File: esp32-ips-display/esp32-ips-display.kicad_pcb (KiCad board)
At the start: 2 copper layers, 25 parts, among them J1 Conn_01x02_Pin, P1 USB_C_Plug_USB2.0, Q1 NPN, Q2 NPN, U1 ESP32-S3-WROOM-1, U2 CH340C, U3 AMS1117-3.3

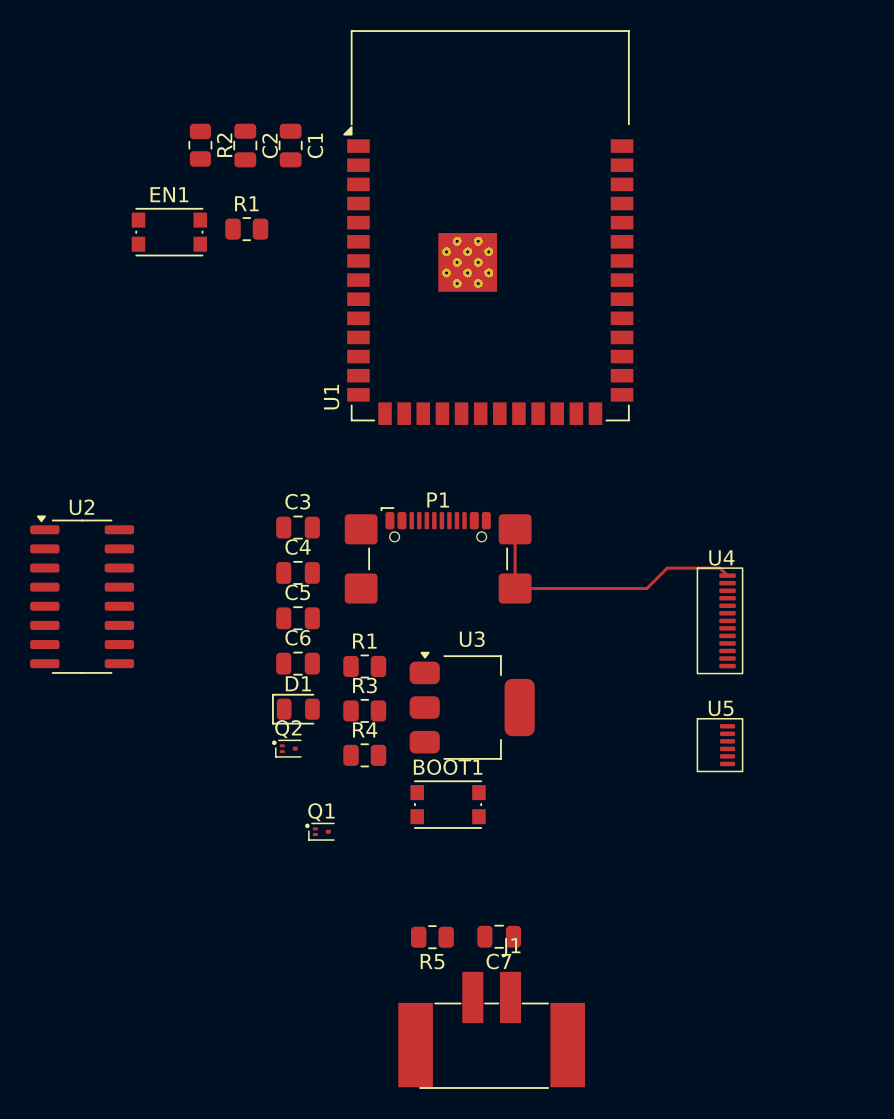
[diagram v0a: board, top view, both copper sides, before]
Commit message: JH
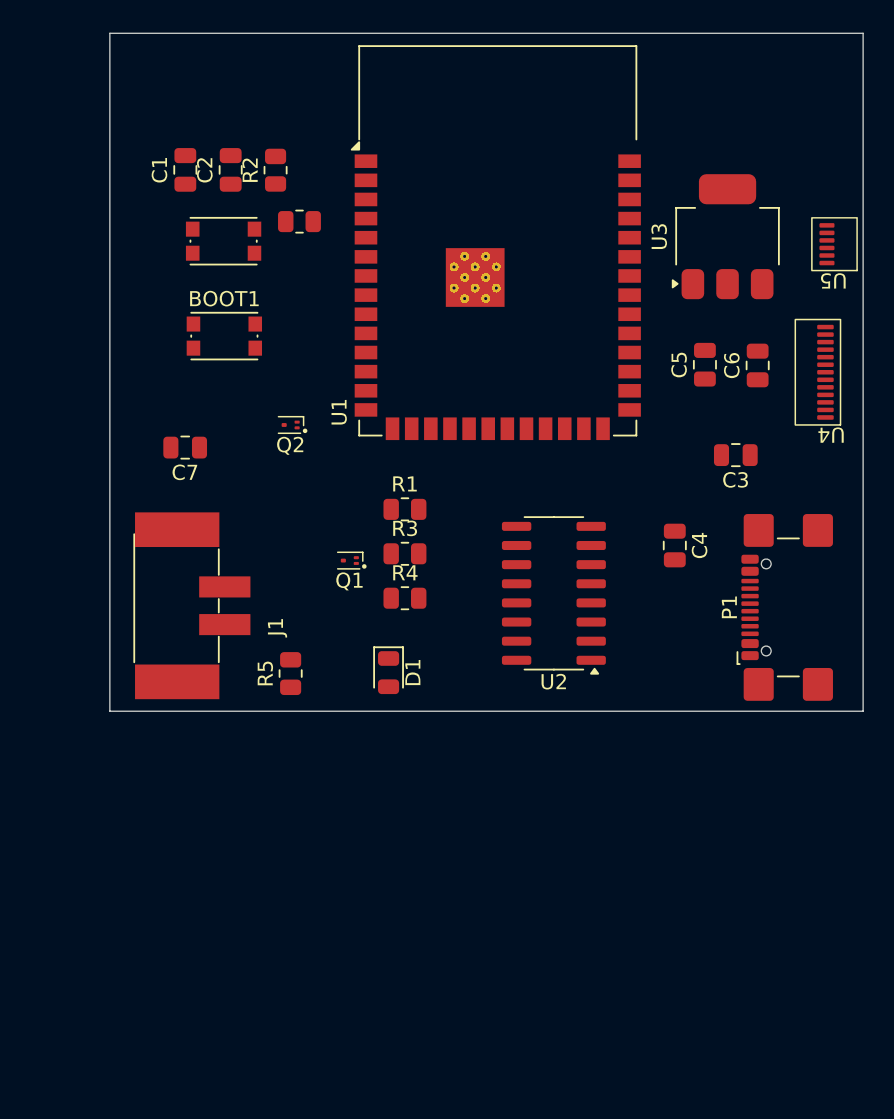
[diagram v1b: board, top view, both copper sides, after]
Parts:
- moved C7 38.6 mm to (145.0, 101.0)
- moved C6 36.4 mm to (183.0, 95.5), turned to 90 degrees
- moved U3 35.6 mm to (181.0, 87.0), turned to 90 degrees
- moved BOOT1 34.5 mm to (147.6, 93.6)
- moved J1 34.4 mm to (145.5, 111.5), turned to 90 degrees
- moved U5 34.1 mm to (186.6, 87.2), turned to 180 degrees
- moved C5 31.8 mm to (179.5, 95.5), turned to 90 degrees
- moved U2 31.3 mm to (169.5, 110.7), turned to 180 degrees
- moved C3 29.5 mm to (181.6, 101.5), turned to 180 degrees
- moved C4 25.1 mm to (177.5, 107.5), turned to -90 degrees
- moved P1 24.5 mm to (186.2, 111.6), turned to 90 degrees
- moved Q2 21.5 mm to (152.0, 99.5), turned to 180 degrees
- moved R5 19.9 mm to (152.0, 116.0), turned to 90 degrees
- moved Q1 18.1 mm to (155.9, 108.5), turned to 180 degrees
- moved U4 17.1 mm to (186.5, 96.0), turned to 180 degrees
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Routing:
- net GND: track 18.8 -> 0.00 mm
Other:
- board outline added: 50 x 45 mm
